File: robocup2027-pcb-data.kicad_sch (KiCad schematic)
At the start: 48 parts, among them M5 Motor_Servo, M6 Motor_Servo, Q1 BPW40, Q2 BPW40, U1 ESP32-DEVKITC-32E

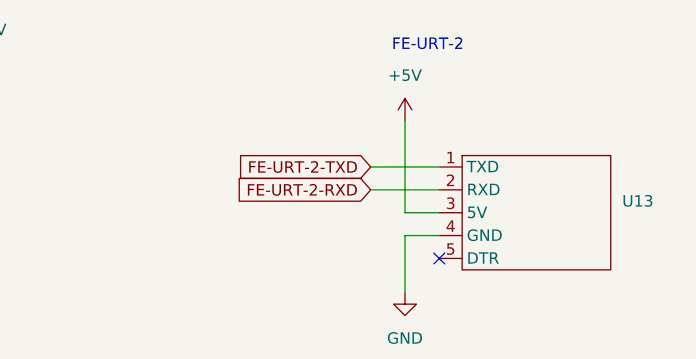
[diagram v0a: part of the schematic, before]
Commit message: finished tracing
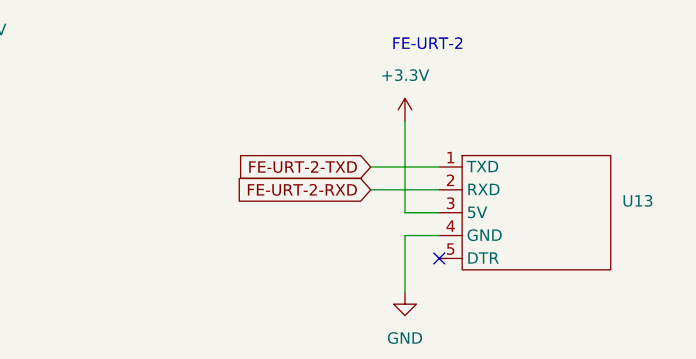
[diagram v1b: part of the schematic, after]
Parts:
- S1, S2: footprint 4-1437565-0:SW_4-1437565-0 -> robo:CW-SB11KKFF
- U1: footprint ESP32-DEVKITC-32E:MODULE_ESP32-DEVKITC-32E -> robo:MODULE_ESP32-DEVKITC-32E
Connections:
- net +3.3V: now also U13.3 (5V)
- net +5V: no longer U13.3 (5V)
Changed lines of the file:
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@@
 	)
 	(symbol
-		(lib_id "power:+5V")
-		(at 303.53 25.4 0)
-		(unit 1)
-		(exclude_from_sim no)
-		(in_bom yes)
-		(on_board yes)
-		(dnp no)
-		(fields_autoplaced yes)
-		(property "Reference" "#PWR025"
-			(at 303.53 29.21 0)
-			(effects
-				(font
-					(size 1.27 1.27)
-				)
-				(hide yes)
-			)
-		)
-		(property "Value" "+5V"
-			(at 303.53 20.32 0)
-			(effects
-				(font
-					(size 1.27 1.27)
-				)
-			)
-		)
-		(property "Footprint" ""
-			(at 303.53 25.4 0)
-			(effects
-				(font
-					(size 1.27 1.27)
-				)
-				(hide yes)
-			)
-		)
-		(property "Datasheet" ""
-			(at 303.53 25.4 0)
-			(effects
-				(font
-					(size 1.27 1.27)
-				)
-				(hide yes)
-			)
-		)
-		(property "Description" "Power symbol creates a global label with name \"+5V\""
-			(at 303.53 25.4 0)
-			(effects
-				(font
-					(size 1.27 1.27)
-				)
-				(hide yes)
-			)
-		)
-		(pin "1"
-		)
-		(instances
-			(project "robocup2027-pcb-data"
-				(path "/fda8bdee-4e79-4e78-9174-7c0702f316a4"
-					(reference "#PWR025")
-					(unit 1)
-				)
-			)
-		)
-	)
-	(symbol
 		(lib_id "Motor:Motor_Servo")
 		(at 134.62 50.8 0)
@@
 			)
 		)
-		(property "Footprint" "ESP32-DEVKITC-32E:MODULE_ESP32-DEVKITC-32E"
+		(property "Footprint" "robo:MODULE_ESP32-DEVKITC-32E"
 			(at 114.3 146.05 0)
 			(effects
@@
 			)
 		)
-		(property "Footprint" "4-1437565-0:SW_4-1437565-0"
+		(property "Footprint" "robo:CW-SB11KKFF"
 			(at 86.36 133.35 0)
 			(effects
@@
 			)
 		)
-		(property "Footprint" "4-1437565-0:SW_4-1437565-0"
+		(property "Footprint" "robo:CW-SB11KKFF"
 			(at 38.1 38.1 0)
 			(effects
@@
 		)
 		(instances
-			(project ""
+			(project "robocup2027-pcb-data"
 				(path "/fda8bdee-4e79-4e78-9174-7c0702f316a4"
 					(reference "U17")
@@
 					(unit 1)
 				)
+			)
+		)
+	)
+	(symbol
+		(lib_id "power:+3.3V")
+		(at 303.53 25.4 0)
+		(unit 1)
+		(exclude_from_sim no)
+		(in_bom yes)
+		(on_board yes)
+		(dnp no)
+		(fields_autoplaced yes)
+		(property "Reference" "#PWR025"
+			(at 303.53 29.21 0)
+			(effects
+				(font
+					(size 1.27 1.27)
+				)
+				(hide yes)
+			)
+		)
+		(property "Value" "+3.3V"
+			(at 303.53 20.32 0)
+			(effects
+				(font
+					(size 1.27 1.27)
+				)
+			)
+		)
+		(property "Footprint" ""
+			(at 303.53 25.4 0)
+			(effects
+				(font
+					(size 1.27 1.27)
+				)
+				(hide yes)
+			)
+		)
+		(property "Datasheet" ""
+			(at 303.53 25.4 0)
+			(effects
+				(font
+					(size 1.27 1.27)
+				)
+				(hide yes)
+			)
+		)
+		(property "Description" "Power symbol creates a global label with name \"+3.3V\""
+			(at 303.53 25.4 0)
+			(effects
+				(font
+					(size 1.27 1.27)
+				)
+				(hide yes)
+			)
+		)
+		(pin "1"
+		)
+		(instances
+			(project "robocup2027-pcb-data"
+				(path "/fda8bdee-4e79-4e78-9174-7c0702f316a4"
+					(reference "#PWR025")
+					(unit 1)
+				)
